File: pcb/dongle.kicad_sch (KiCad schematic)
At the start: 32 parts, among them J1 USB_A, J2 Conn_01x01_Pin, J3 Conn_01x01_Pin, J4 Conn_01x01_Pin, J5 Conn_01x01_Pin, U3 nRF52833_QDxx, Y1 Crystal_GND24, Y2 Crystal_Small

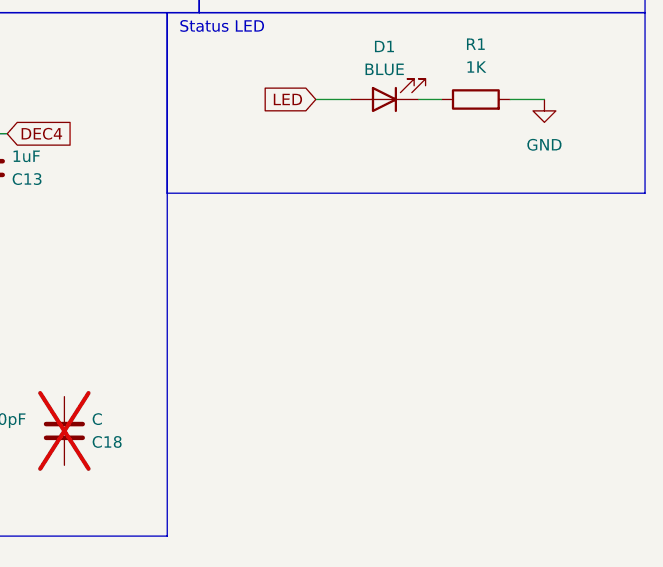
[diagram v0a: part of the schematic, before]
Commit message: update pcb
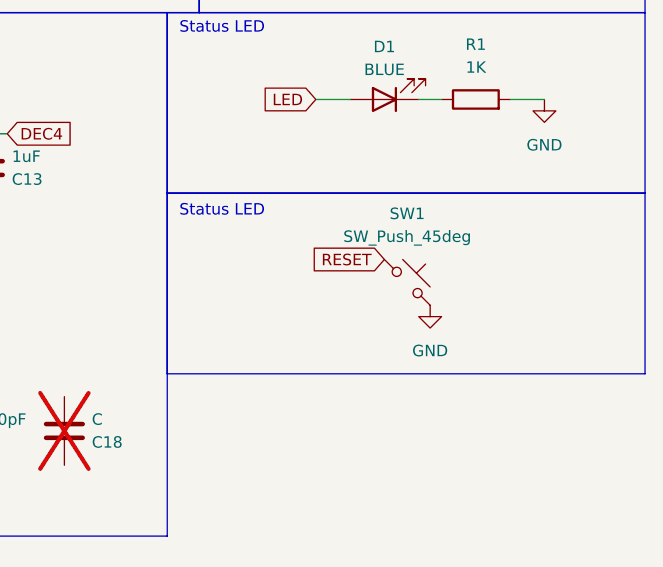
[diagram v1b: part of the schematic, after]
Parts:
- added SW1: SW_Push_45deg, dongle:SKTAAAE010, symbol dongle:SW_Push_45deg
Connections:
- net GND: now also SW1.2
- net RESET: now also SW1.1
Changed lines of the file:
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@@
 		)
 	)
+	(rectangle
+		(start 231.14 73.914)
+		(end 284.226 93.98)
+		(stroke
+			(width 0)
+			(type default)
+		)
+		(fill
+			(type none)
+		)
+	)
 	(text "USB"
 		(exclude_from_sim no)
@@
 		)
 	)
+	(text "Status LED"
+		(exclude_from_sim no)
+		(at 237.236 75.946 0)
+		(effects
+			(font
+				(size 1.27 1.27)
+			)
+		)
+	)
 	(text "XTAL"
 		(exclude_from_sim no)
@@
 		)
 	)
+	(global_label "RESET"
+		(shape input)
+		(at 255.27 81.28 180)
+		(fields_autoplaced yes)
+		(effects
+			(font
+				(size 1.27 1.27)
+			)
+			(justify right)
+		)
+		(property "Intersheetrefs" "${INTERSHEET_REFS}"
+			(at 246.5397 81.28 0)
+			(effects
+				(font
+					(size 1.27 1.27)
+				)
+				(justify right)
+				(hide yes)
+			)
+		)
+	)
 	(global_label "D+"
 		(shape input)
@@
 	)
 	(symbol
+		(lib_id "Library:GND")
+		(at 260.35 86.36 0)
+		(unit 1)
+		(exclude_from_sim no)
+		(in_bom yes)
+		(on_board yes)
+		(dnp no)
+		(fields_autoplaced yes)
+		(property "Reference" "#PWR05"
+			(at 260.35 92.71 0)
+			(effects
+				(font
+					(size 1.27 1.27)
+				)
+				(hide yes)
+			)
+		)
+		(property "Value" "GND"
+			(at 260.35 91.44 0)
+			(effects
+				(font
+					(size 1.27 1.27)
+				)
+			)
+		)
+		(property "Footprint" ""
+			(at 260.35 86.36 0)
+			(effects
+				(font
+					(size 1.27 1.27)
+				)
+				(hide yes)
+			)
+		)
+		(property "Datasheet" ""
+			(at 260.35 86.36 0)
+			(effects
+				(font
+					(size 1.27 1.27)
+				)
+				(hide yes)
+			)
+		)
+		(property "Description" "Global ground symbol"
+			(at 260.35 95.758 0)
+			(effects
+				(font
+					(size 1.27 1.27)
+				)
+				(hide yes)
+			)
+		)
+		(pin "1"
+		)
+		(instances
+			(project "dongle"
+				(path "/81b8789c-509b-48aa-aabd-6327c54a25df"
+					(reference "#PWR05")
+					(unit 1)
+				)
+			)
+		)
+	)
+	(symbol
 		(lib_id "PNCATEHO_lowair:C")
 		(at 219.71 100.33 0)
@@
 					(unit 1)
 				)
+			)
+		)
+	)
+	(symbol
+		(lib_id "dongle:SW_Push_45deg")
+		(at 257.81 83.82 0)
+		(unit 1)
+		(exclude_from_sim no)
+		(in_bom yes)
+		(on_board yes)
+		(dnp no)
+		(fields_autoplaced yes)
+		(property "Reference" "SW1"
+			(at 257.81 76.2 0)
+			(effects
+				(font
+					(size 1.27 1.27)
+				)
+			)
+		)
+		(property "Value" "SW_Push_45deg"
+			(at 257.81 78.74 0)
+			(effects
+				(font
+					(size 1.27 1.27)
+				)
+			)
+		)
+		(property "Footprint" "dongle:SKTAAAE010"
+			(at 257.81 83.82 0)
+			(effects
+				(font
+					(size 1.27 1.27)
+				)
+				(hide yes)
+			)
+		)
+		(property "Datasheet" "~"
+			(at 257.81 83.82 0)
+			(effects
+				(font
+					(size 1.27 1.27)
+				)
+				(hide yes)
+			)
+		)
+		(property "Description" "Push button switch, normally open, two pins, 45° tilted"
+			(at 257.81 83.82 0)
+			(effects
+				(font
+					(size 1.27 1.27)
+				)
+				(hide yes)
+			)
+		)
+		(pin "2"
+		)
+		(pin "1"
+		)
+		(instances
+			(project ""
+				(path "/81b8789c-509b-48aa-aabd-6327c54a25df"
+					(reference "SW1")
+					(unit 1)
+				)

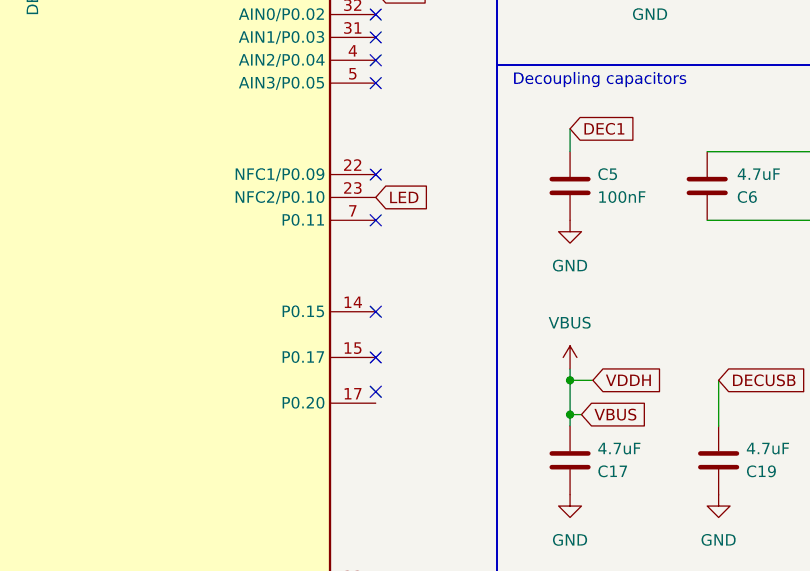
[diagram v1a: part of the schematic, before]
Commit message: fix routing
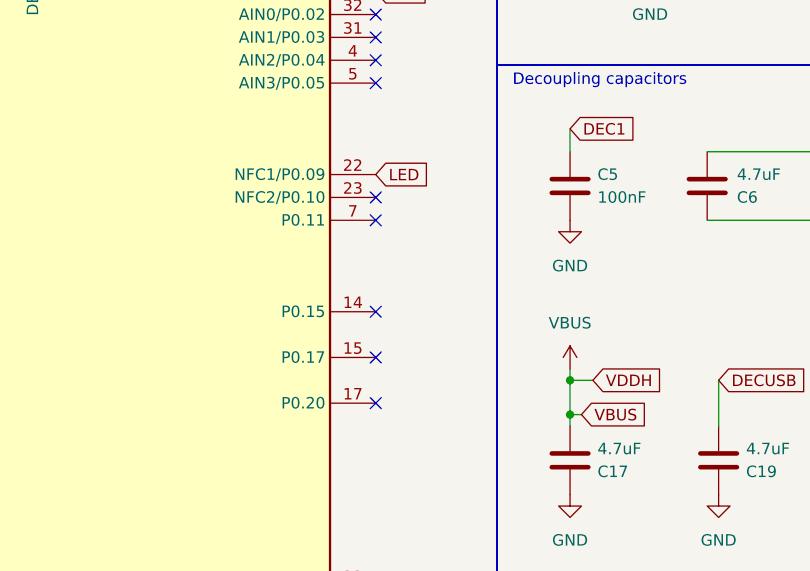
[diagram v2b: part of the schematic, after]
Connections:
- net LED: now also U3.22 (NFC1/P0.09); no longer U3.23 (NFC2/P0.10)
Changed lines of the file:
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@@
+	)
+	(no_connect
+		(at 92.71 68.58)
 	)
 	(no_connect
@@
 	)
 	(no_connect
+		(at 92.71 91.44)
+	)
+	(no_connect
 		(at 92.71 86.36)
 	)
 	(no_connect
-		(at 92.71 90.17)
-	)
-	(no_connect
 		(at 92.71 114.3)
 	)
@@
 	)
 	(no_connect
-		(at 92.71 66.04)
-	)
-	(no_connect
 		(at 49.53 35.56)
 	)
@@
 	(global_label "LED"
 		(shape input)
-		(at 92.71 68.58 0)
-		(fields_autoplaced yes)
-		(effects
-			(font
-				(size 1.27 1.27)
-			)
-			(justify left)
-		)
-		(property "Intersheetrefs" "${INTERSHEET_REFS}"
-			(at 99.1423 68.58 0)
-			(effects
-				(font
+		(at 92.71 66.04 0)
+		(fields_autoplaced yes)
+		(effects
+			(font
+				(size 1.27 1.27)
+			)
+			(justify left)
+		)
+		(property "Intersheetrefs" "${INTERSHEET_REFS}"
+			(at 99.1423 66.04 0)
+			(effects
+				(font
